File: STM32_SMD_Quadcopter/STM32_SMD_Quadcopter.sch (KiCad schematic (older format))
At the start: 61 parts, among them J1 PWR, J2 USB_B_Micro, J3 Micro_SD_Card, J4 DEBUG, J5 DSMX, M1 Brushed_DC, M2 Brushed_DC, M3 Brushed_DC, M4 Brushed_DC, Q1 IRLML6244TR, Q2 IRLML6244TR, Q3 IRLML6244TR, Q4 IRLML6244TR, SW1 SW_Push, U1 LT1129-3.3_SOT223, U2 MPU-9250, U3 FT230XQ, U4 STM32F446RETx, Y1 8MHz ECS801830JGNTR

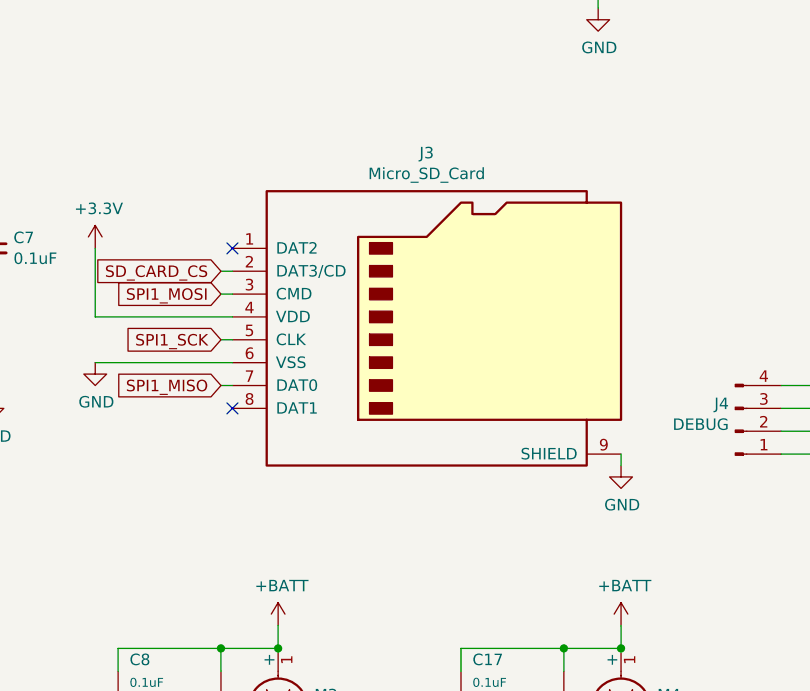
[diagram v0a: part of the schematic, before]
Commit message: Completed board v1
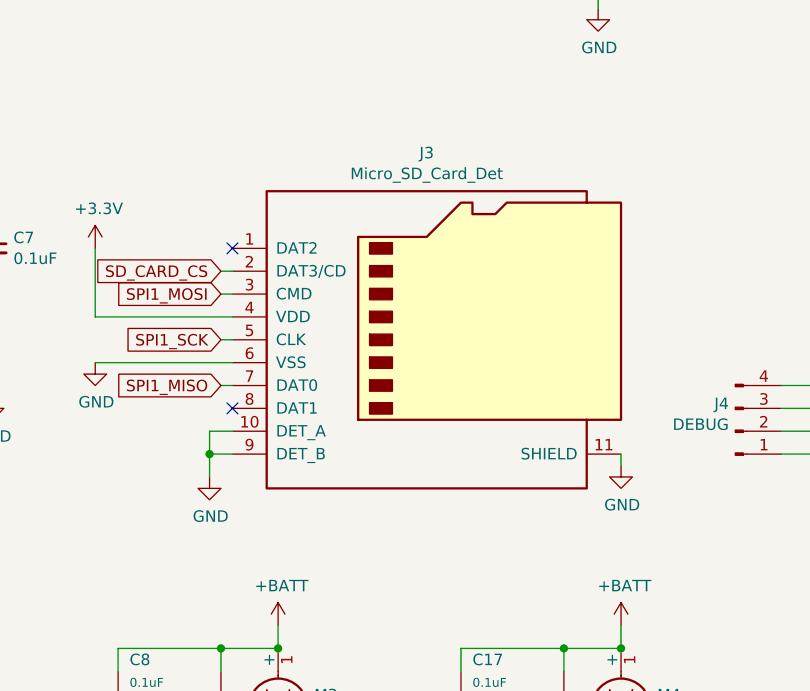
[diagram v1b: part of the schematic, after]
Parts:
- removed J3: Micro_SD_Card, Connector_Card:microSD_HC_Hirose_DM3D-SF, symbol STM32_SMD_Quadcopter-rescue:Micro_SD_Card-Connector
- added J3: Micro_SD_Card_Det, Connector_Card:microSD_HC_Hirose_DM3D-SF, symbol Connector:Micro_SD_Card_Det
- J4: footprint Connector_PinHeader_2.54mm:PinHeader_1x04_P2.54mm_Vertical -> Connector_Harwin:Harwin_M20-89004xx_1x04_P2.54mm_Horizontal
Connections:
- net +3V3: now also J3.4 (VDD)
- net GND: now also J3.10 (DET_A), J3.11 (SHIELD), J3.6 (VSS), J3.9 (DET_B)
- net SD_CARD_CS: now also J3.2 (DAT3/CD)
- net SPI1_MISO: now also J3.7 (DAT0)
- net SPI1_MOSI: now also J3.3 (CMD)
- net SPI1_SCK: now also J3.5 (CLK)
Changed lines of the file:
@@
 	900  3000 950  3000
-$Comp
-L STM32_SMD_Quadcopter-rescue:Micro_SD_Card-Connector J3
-U 1 1 5D1D8D5D
-P 5200 5000
-F 0 "J3" H 5150 5717 50  0000 C CNN
-F 1 "Micro_SD_Card" H 5150 5626 50  0000 C CNN
-F 2 "Connector_Card:microSD_HC_Hirose_DM3D-SF" H 6350 5300 50  0001 C CNN
-F 3 "http://katalog.we-online.de/em/datasheet/693072010801.pdf" H 5200 5000 50  0001 C CNN
-	1    5200 5000
-	1    0    0    -1
-$EndComp
 $Comp
 L Connector:USB_B_Micro J2
@@
 F 0 "J4" H 6472 5380 50  0000 R CNN
 F 1 "DEBUG" H 6472 5471 50  0000 R CNN
-F 2 "Connector_PinHeader_2.54mm:PinHeader_1x04_P2.54mm_Vertical" H 6500 5500 50  0001 C CNN
+F 2 "Connector_Harwin:Harwin_M20-89004xx_1x04_P2.54mm_Horizontal" H 6500 5500 50  0001 C CNN
 F 3 "~" H 6500 5500 50  0001 C CNN
 	1    6500 5500
@@
 	9750 5450 9700 5450
 NoConn ~ 8300 5150
+$Comp
+L Connector:Micro_SD_Card_Det J3
+U 1 1 5EAFBA60
+P 5200 5100
+F 0 "J3" H 5150 5917 50  0000 C CNN
+F 1 "Micro_SD_Card_Det" H 5150 5826 50  0000 C CNN
+F 2 "Connector_Card:microSD_HC_Hirose_DM3D-SF" H 7250 5800 50  0001 C CNN
+F 3 "https://www.hirose.com/product/en/download_file/key_name/DM3/category/Catalog/doc_file_id/49662/?file_category_id=4&item_id=195&is_series=1" H 5200 5200 50  0001 C CNN
+	1    5200 5100
+	1    0    0    -1
+$EndComp
+$Comp
+L power:GND #PWR?
+U 1 1 5EB10C43
+P 4200 5700
+F 0 "#PWR?" H 4200 5450 50  0001 C CNN
+F 1 "GND" H 4205 5527 50  0000 C CNN
+F 2 "" H 4200 5700 50  0001 C CNN
+F 3 "" H 4200 5700 50  0001 C CNN
+	1    4200 5700
+	1    0    0    -1
+$EndComp
+Wire Wire Line
+	4200 5700 4200 5600
+Wire Wire Line
+	4200 5600 4300 5600
+Wire Wire Line
+	4300 5500 4200 5500
+Wire Wire Line
+	4200 5500 4200 5600
+Connection ~ 4200 5600
 $EndSCHEMATC
